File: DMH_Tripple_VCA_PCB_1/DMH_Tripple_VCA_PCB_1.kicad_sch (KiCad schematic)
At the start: 0 parts

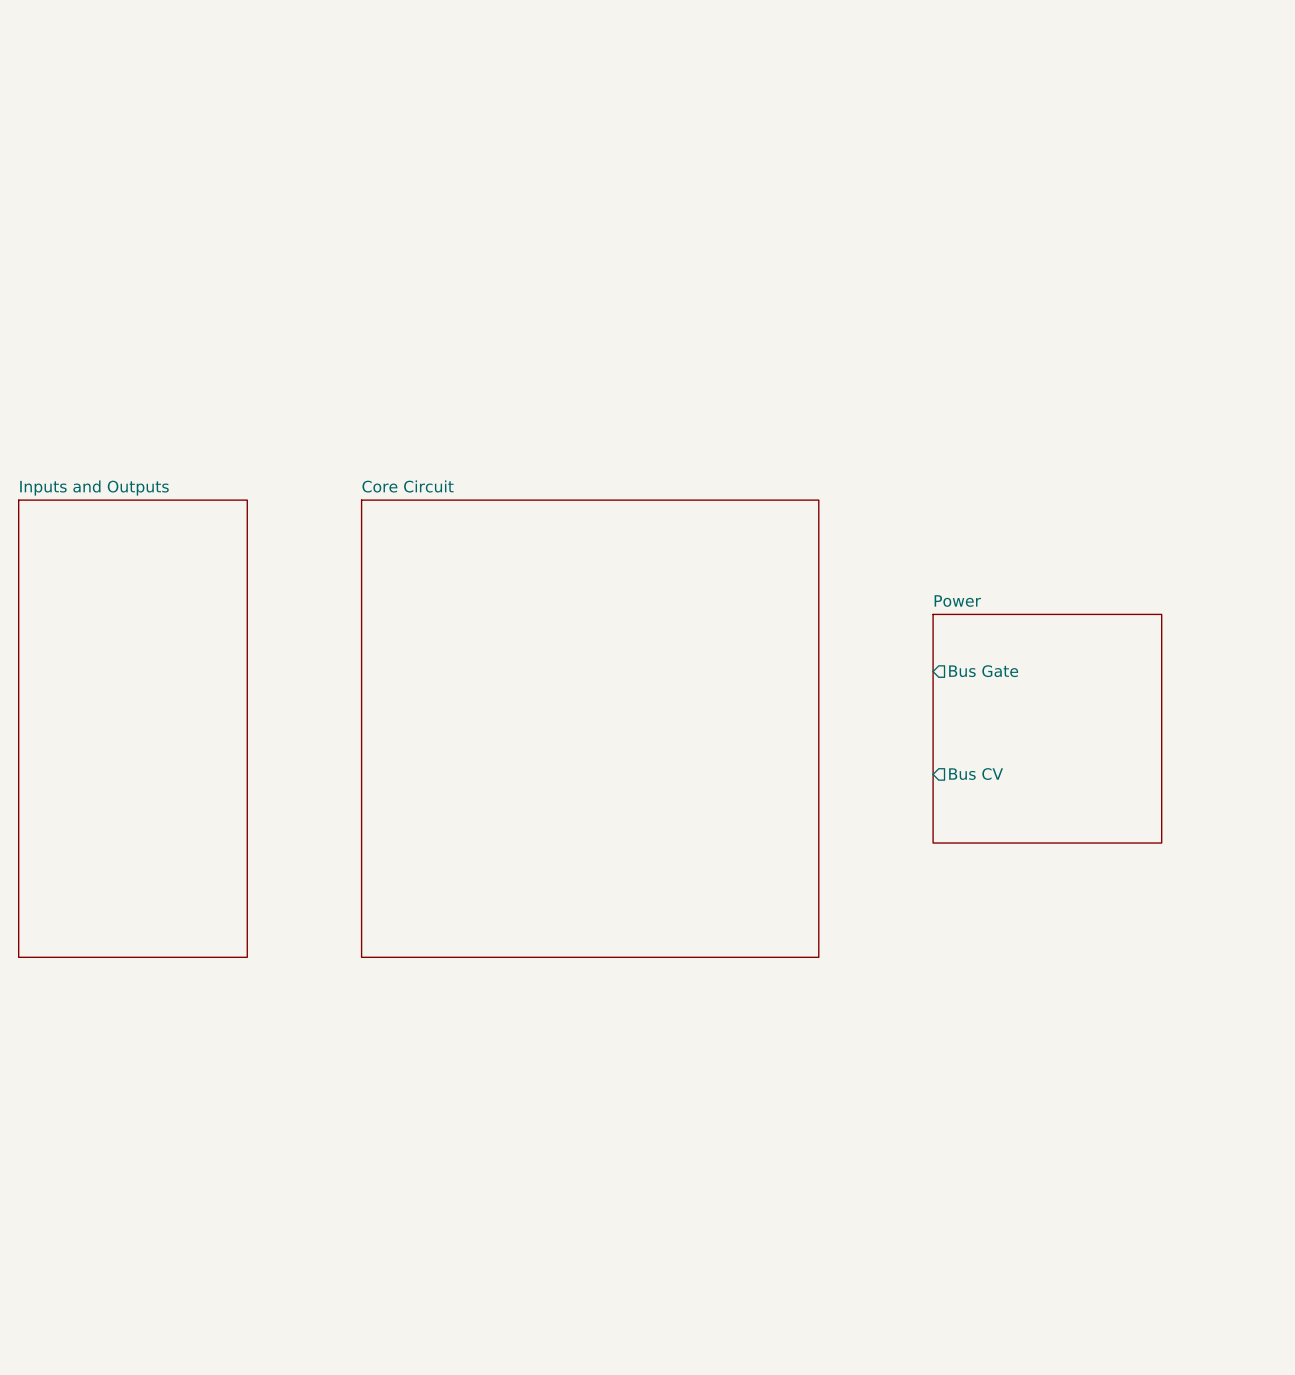
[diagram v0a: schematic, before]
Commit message: Schematic in progress
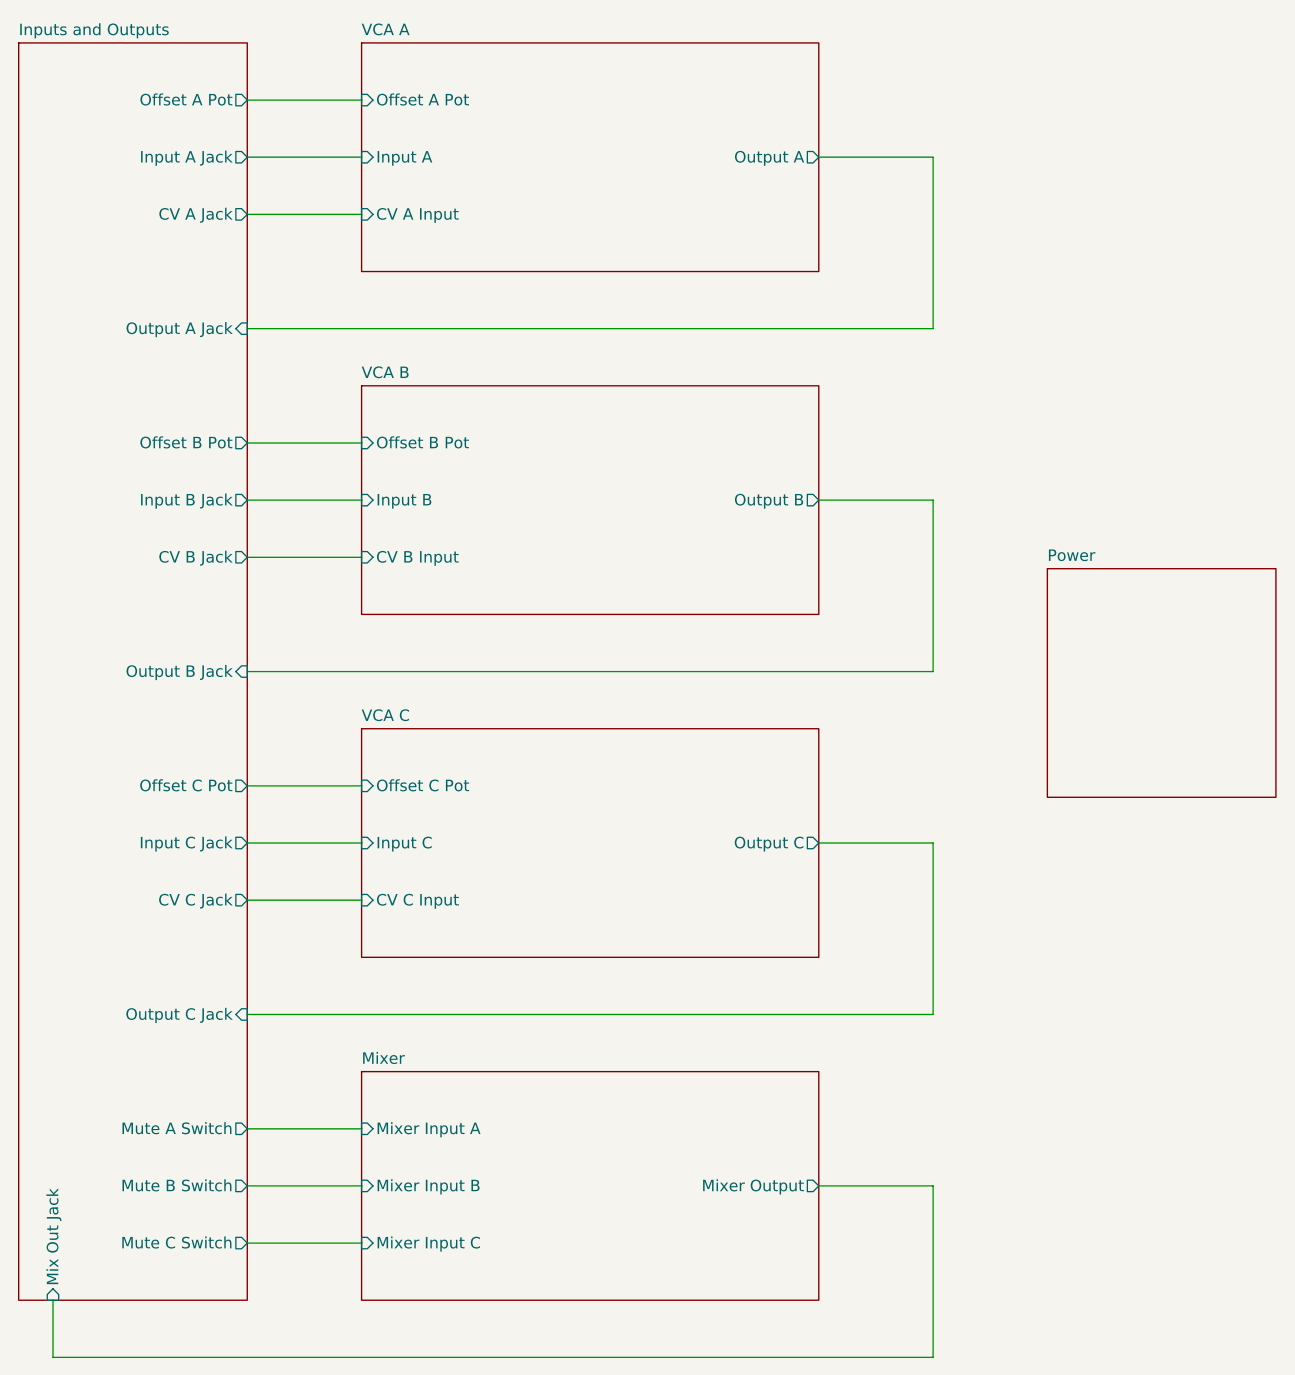
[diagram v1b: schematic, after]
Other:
- sheet Core Circuit renamed VCA A
- added sheet Mixer (Mixer.kicad_sch)
- added sheet VCA B (VCA_B.kicad_sch)
- added sheet VCA C (VCA_C.kicad_sch)
- sheet Inputs and Outputs ports: added CV A Jack, CV B Jack, CV C Jack, Input A Jack, Input B Jack, Input C Jack, Mix Out Jack, Mute A Switch, Mute B Switch, Mute C Switch, Offset A Pot, Offset B Pot, Offset C Pot, Output A Jack, Output B Jack, Output C Jack; removed none
- sheet Power ports: added none; removed Bus CV, Bus Gate
- sheet VCA A: file Core_Circuit.kicad_sch -> VCA_A.kicad_sch
- sheet VCA A ports: added CV A Input, Input A, Offset A Pot, Output A; removed none
